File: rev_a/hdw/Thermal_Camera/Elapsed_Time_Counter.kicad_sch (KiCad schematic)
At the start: 7 parts

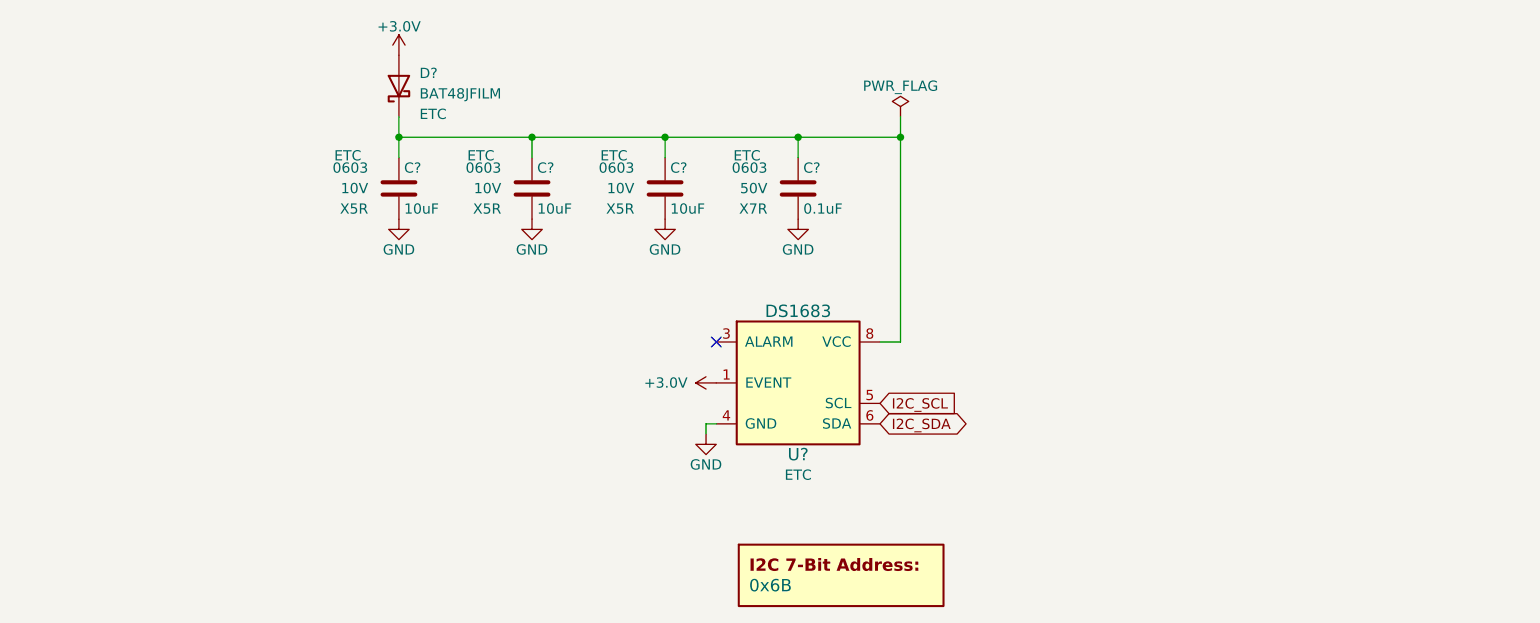
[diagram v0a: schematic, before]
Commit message: added some more USB stuff
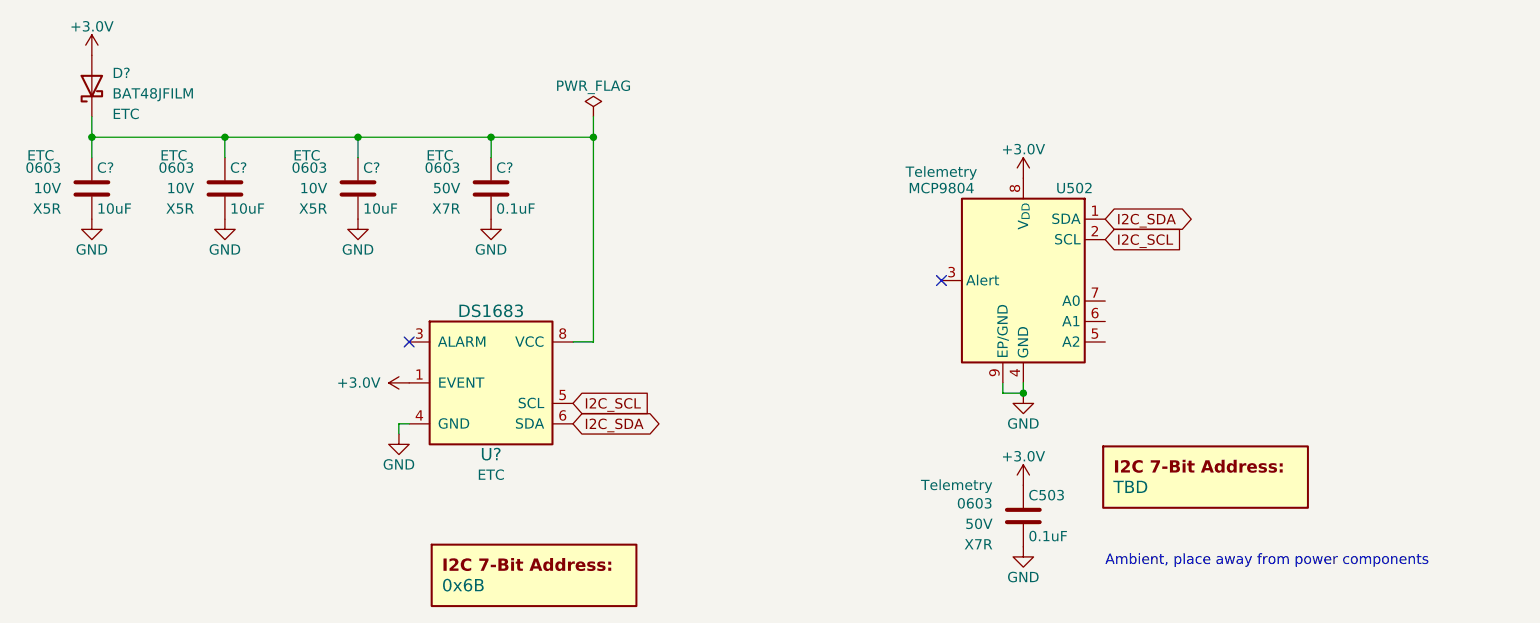
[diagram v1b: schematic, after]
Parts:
- added C503: 0.1uF, Capacitors_SMD:C_0603, symbol Custom_Library:C_Custom
- added DOC502: TBD, symbol Custom_Library:I2C_Address
- added U502: MCP9804, Package_DFN_QFN:DFN-8-1EP_3x2mm_P0.5mm_EP1.3x1.5mm, symbol Sensor_Temperature:MCP9804_DFN
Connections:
- net +3.0V: now also C503.1, U502.8 (V_{DD})
- net GND: now also C503.2, U502.4 (GND), U502.9 (EP/GND)
- net I2C_SCL: now also U502.2 (SCL)
- net I2C_SDA: now also U502.1 (SDA)
- no-connect marks 1 -> 2
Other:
- note added: "Ambient, place away from power components"
- moved on the sheet: C?, D?, U?
